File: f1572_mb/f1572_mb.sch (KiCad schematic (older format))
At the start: 24 parts, among them Q1 2N3904, SW1 power, SW2 ~reset, U1 PIC12F1572

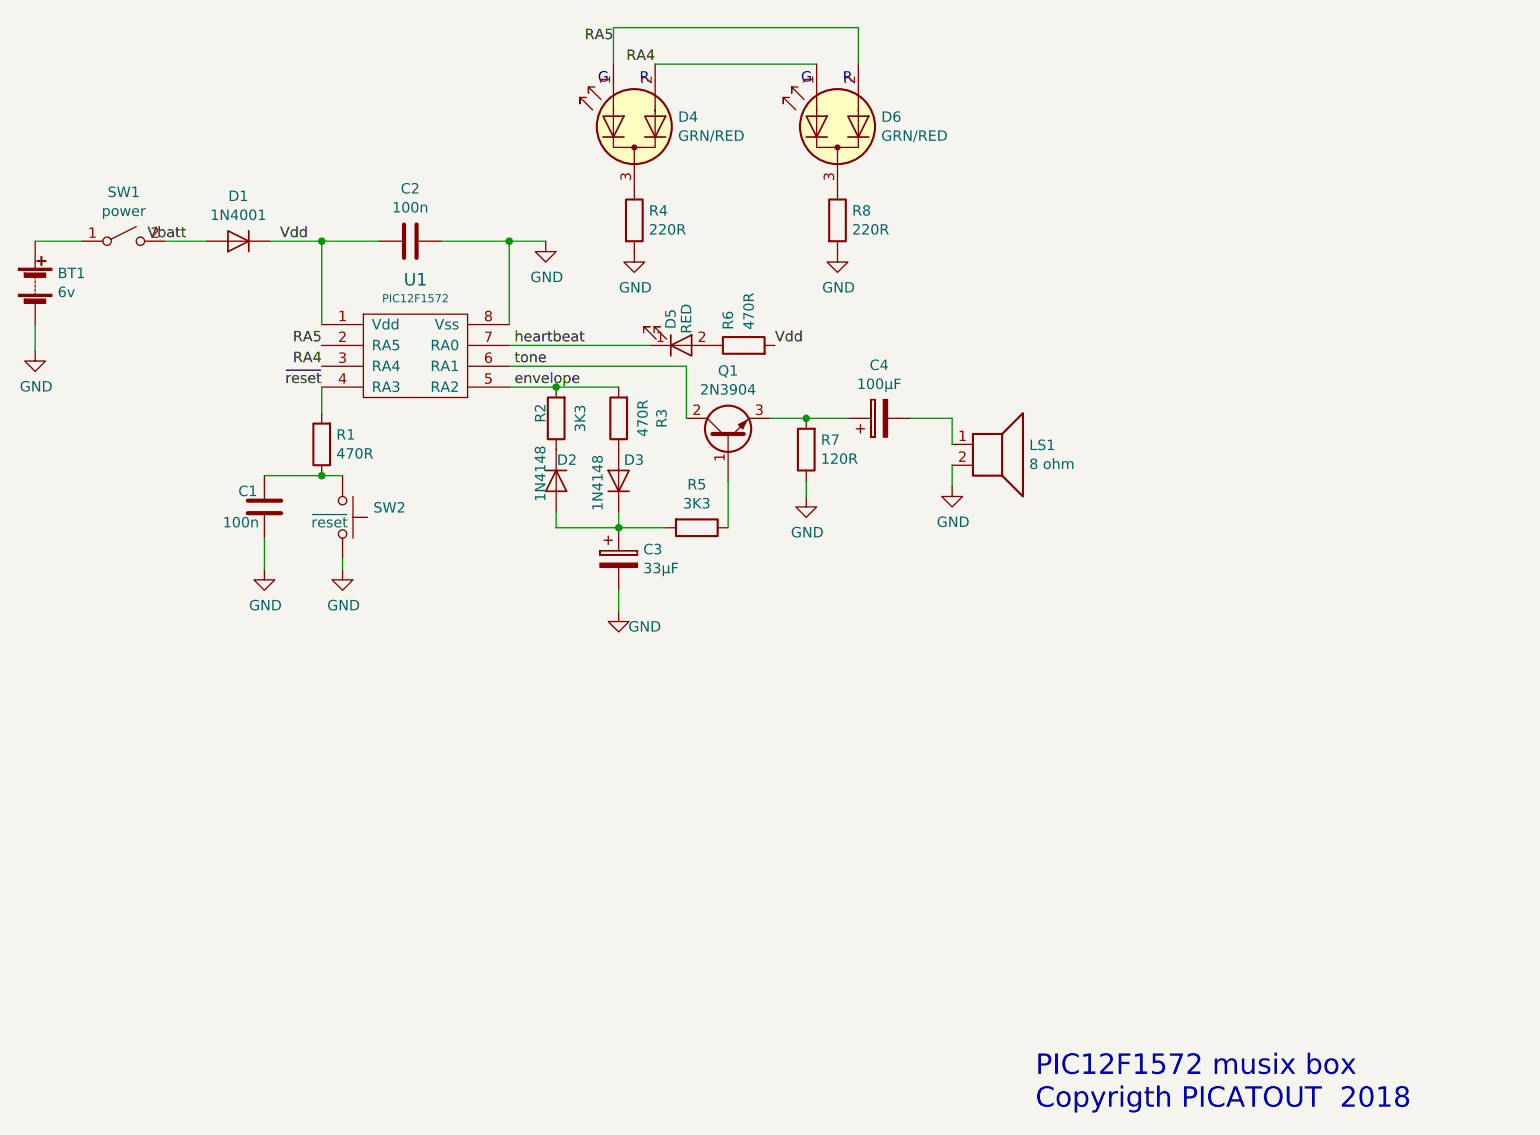
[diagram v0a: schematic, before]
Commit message: Create v2 folder and copied project file to this folder. Modified schematic
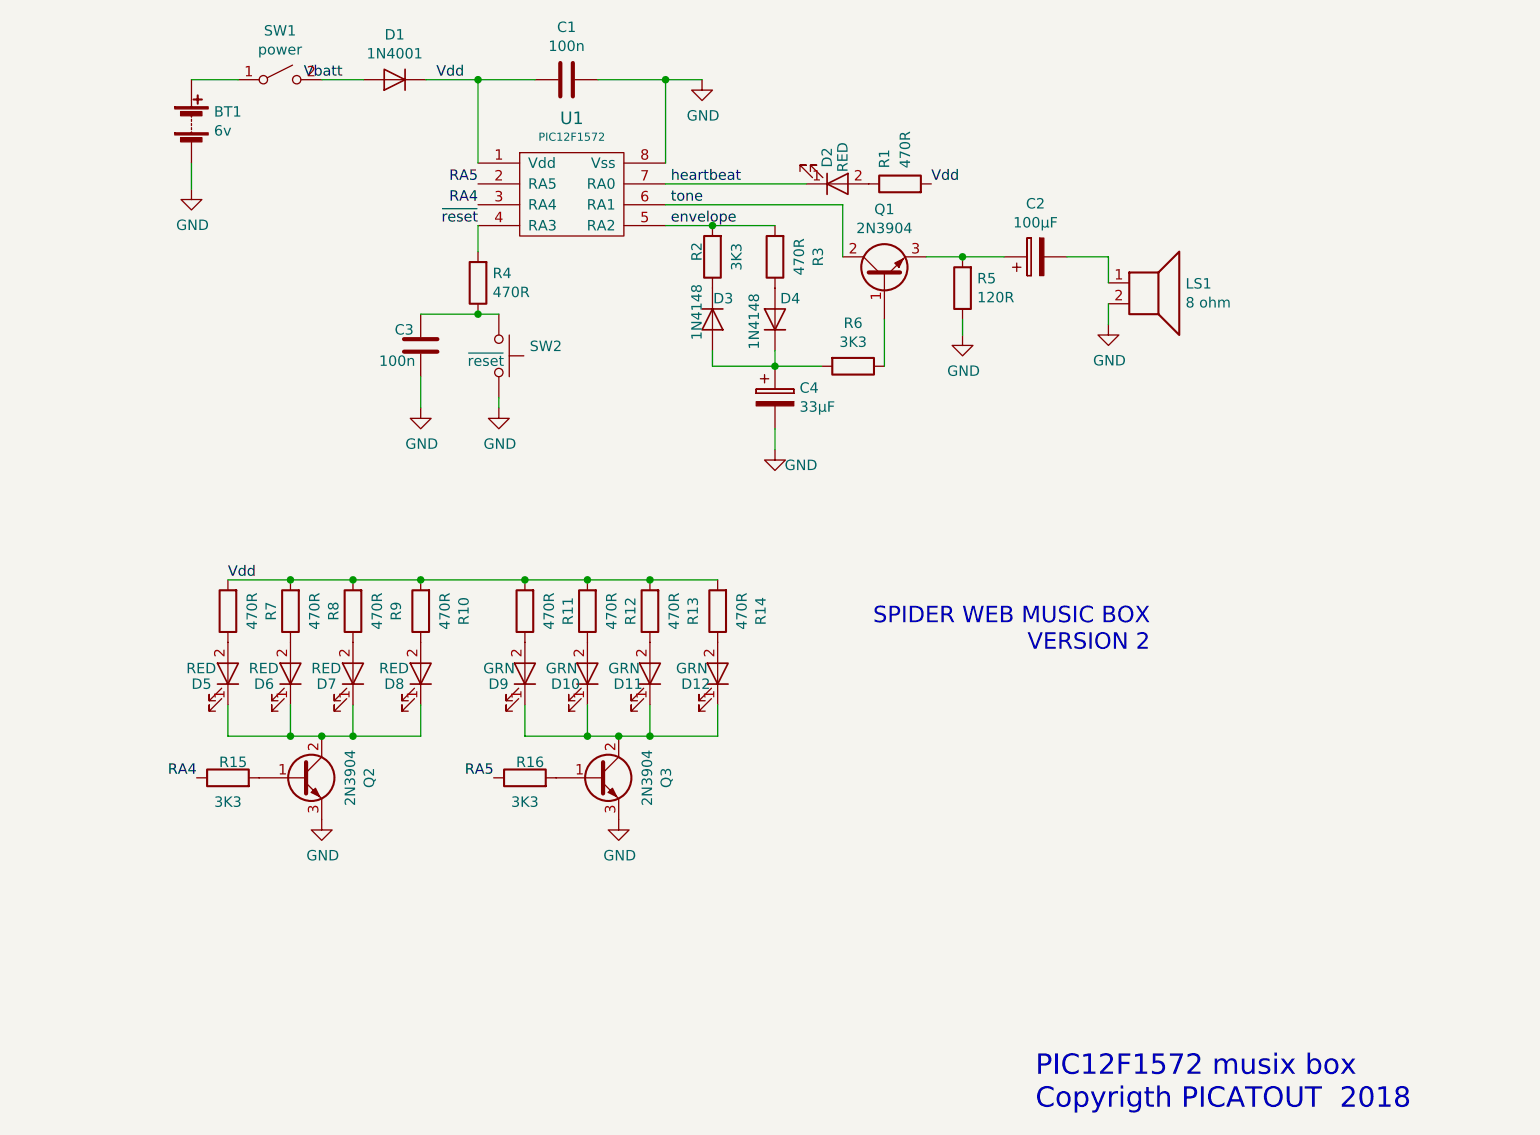
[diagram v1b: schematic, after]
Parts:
- removed D4, D6: GRN/RED, symbol device:LED_Dual_AAC
- removed R4: 220R, symbol device:R
- added D10, D11, D12, D9: GRN, symbol device:LED
- added D5, D6, D7, D8: RED, symbol device:LED
- added Q2, Q3: 2N3904, symbol device:Q_NPN_BCE
- added R10, R11, R12, R13, R14, R7, R9: 470R, symbol device:R
- added R15, R16: 3K3, symbol device:R
- R8: value 220R -> 470R
- renumbered C2 to C1, C4 to C2, C1 to C3, C3 to C4, D5 to D2, D2 to D3, D3 to D4, R6 to R1, R1 to R4, R7 to R5, R5 to R6
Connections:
- net GND: now also Q2.3 (E), Q3.3 (E); no longer R8.2
- net RA4: now also R15.1
- net RA5: now also R16.1
- net Vdd: now also R8.2, R10.2, R11.2, R12.2, R13.2, R14.2, R7.2, R9.2
- net at R8.1: now also D6.2 (A)
- new net: D5.1 (K), D6.1 (K), D7.1 (K), D8.1 (K), Q2.2 (C)
- new net: D5.2 (A), R7.1
- new net: D7.2 (A), R9.1
- new net: D8.2 (A), R10.1
- new net: D10.1 (K), D11.1 (K), D12.1 (K), D9.1 (K), Q3.2 (C)
- new net: D9.2 (A), R11.1
- new net: D10.2 (A), R12.1
- new net: D11.2 (A), R13.1
- new net: D12.2 (A), R14.1
- new net: Q2.1 (B), R15.2
- new net: Q3.1 (B), R16.2
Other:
- note added: "SPIDER WEB MUSIC BOX\nVERSION 2"
- note removed: "G\n"
- note removed: "R"
- moved on the sheet: BT1, C1, C2, C3, C4, D1, D2, D3, D4, LS1, Q1, R1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

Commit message: added png of schematic, updated readme.md
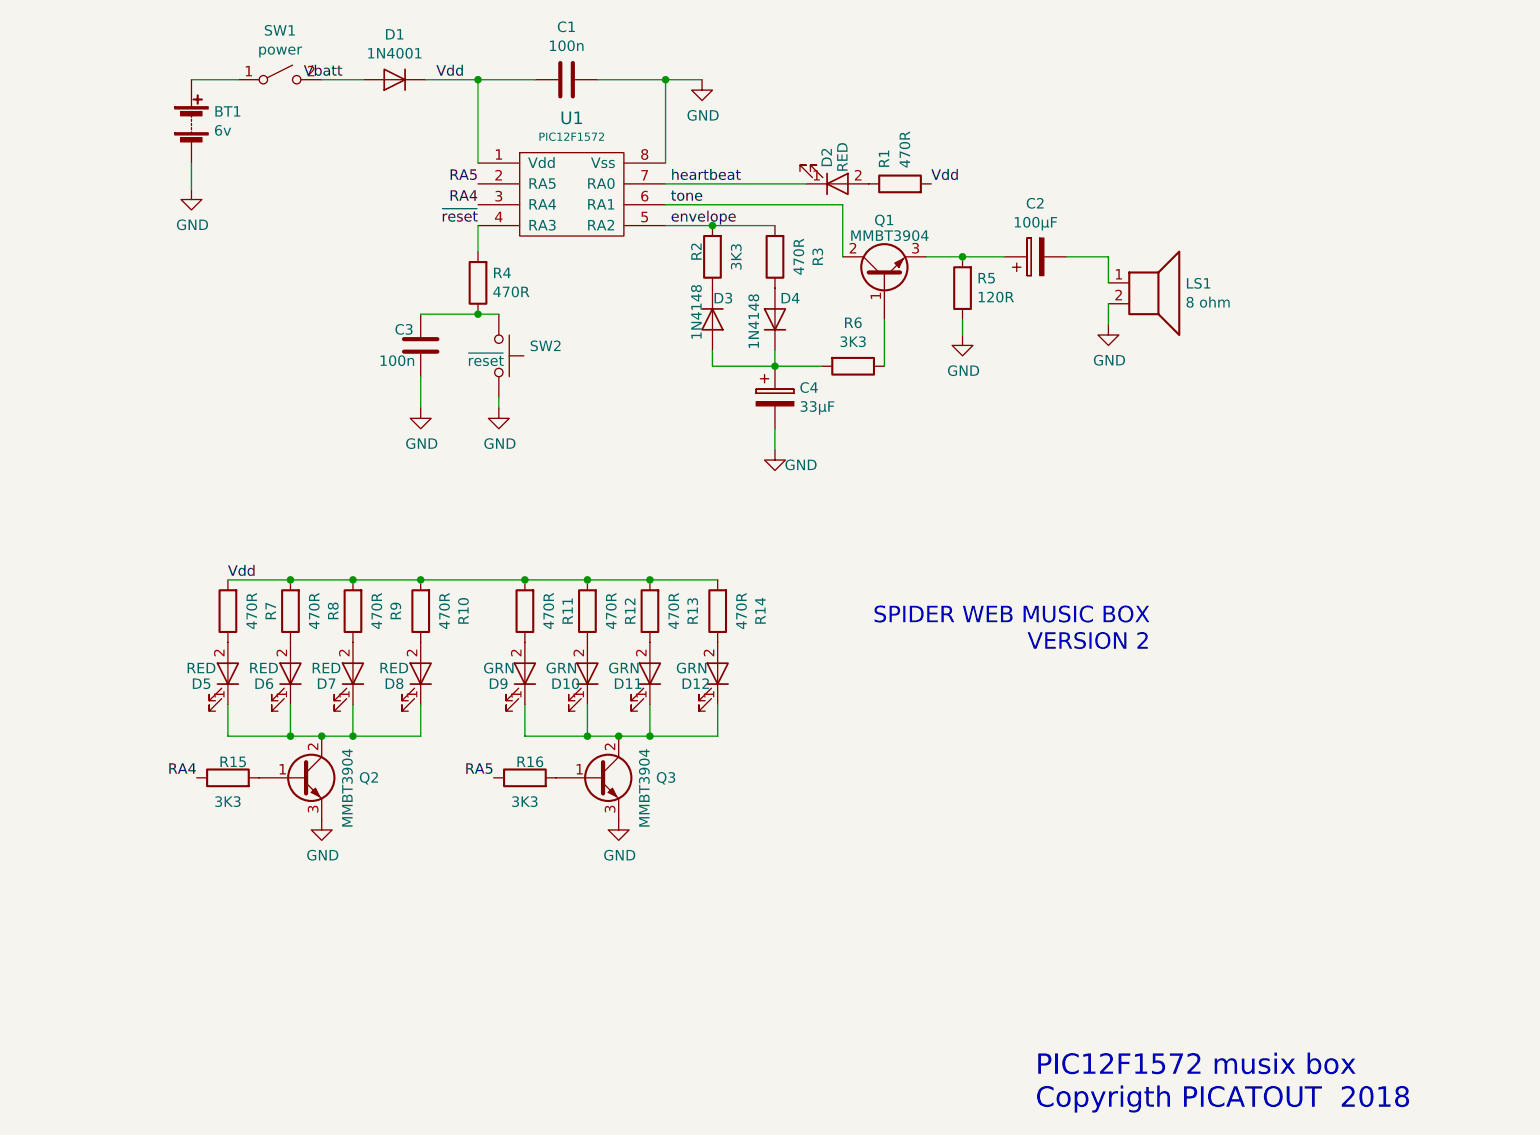
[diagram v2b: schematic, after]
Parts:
- Q1, Q2, Q3: value 2N3904 -> MMBT3904
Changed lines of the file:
@@
 U 1 1 5C074016
 P 6550 2950
-F 0 "Q1" V 6878 2950 50  0000 C CNN
-F 1 "2N3904" V 6787 2950 50  0000 C CNN
+F 0 "Q1" V 6825 2950 50  0000 C CNN
+F 1 "MMBT3904" V 6750 2925 50  0000 C CNN
 F 2 "" H 6750 3050 50  0001 C CNN
 F 3 "" H 6550 2950 50  0001 C CNN
@@
 U 1 1 5C1B7C84
 P 3750 5350
-F 0 "Q2" V 4078 5350 50  0000 C CNN
-F 1 "2N3904" V 3987 5350 50  0000 C CNN
+F 0 "Q2" H 4078 5350 50  0000 C CNN
+F 1 "MMBT3904" V 3975 5300 50  0000 C CNN
 F 2 "" H 3950 5450 50  0001 C CNN
 F 3 "" H 3750 5350 50  0001 C CNN
@@
 U 1 1 5C1B7F86
 P 5175 5350
-F 0 "Q3" V 5503 5350 50  0000 C CNN
-F 1 "2N3904" V 5412 5350 50  0000 C CNN
+F 0 "Q3" H 5503 5350 50  0000 C CNN
+F 1 "MMBT3904" V 5400 5300 50  0000 C CNN
 F 2 "" H 5375 5450 50  0001 C CNN
 F 3 "" H 5175 5350 50  0001 C CNN

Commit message: added photos project completed
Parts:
- C1, C3: footprint (none) -> Capacitors_SMD:C_0805
- D1, D3, D4, R3: footprint (none) -> Diodes_SMD:D_0805
- D10, D11, D12, D2, D5, D6, D7, D8, D9: footprint (none) -> LEDs:LED_0805
- Q1, Q2, Q3: footprint (none) -> TO_SOT_Packages_SMD:SOT-23
- R1, R10, R11, R12, R13, R14, R15, R16, R2, R5, R6, R7, R8, R9: footprint (none) -> Resistors_SMD:R_0805
- R4: footprint (none) -> Resistors_SMD:R_1206
- U1: footprint (none) -> SMD_Packages:SOIC-8-N
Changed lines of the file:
@@
 F 0 "U1" H 5050 2915 60  0000 C CNN
 F 1 "PIC12F1572" H 5050 2825 39  0000 C CNN
-F 2 "" H 5050 2350 60  0001 C CNN
+F 2 "SMD_Packages:SOIC-8-N" H 5050 2350 60  0001 C CNN
 F 3 "" H 5050 2350 60  0001 C CNN
 	1    5050 2550
@@
 F 0 "C1" V 4773 2000 50  0000 C CNN
 F 1 "100n" V 4864 2000 50  0000 C CNN
-F 2 "" H 5063 1850 50  0001 C CNN
+F 2 "Capacitors_SMD:C_0805" H 5063 1850 50  0001 C CNN
 F 3 "" H 5025 2000 50  0001 C CNN
 	1    5025 2000
@@
 F 0 "Q1" V 6825 2950 50  0000 C CNN
 F 1 "MMBT3904" V 6750 2925 50  0000 C CNN
-F 2 "" H 6750 3050 50  0001 C CNN
+F 2 "TO_SOT_Packages_SMD:SOT-23" H 6750 3050 50  0001 C CNN
 F 3 "" H 6550 2950 50  0001 C CNN
 	1    6550 2950
@@
 F 0 "R5" H 6855 2954 50  0000 R CNN
 F 1 "120R" H 6855 3045 50  0000 R CNN
-F 2 "" V 6855 3000 50  0001 C CNN
+F 2 "Resistors_SMD:R_0805" V 6855 3000 50  0001 C CNN
 F 3 "" H 6925 3000 50  0001 C CNN
 	1    6925 3000
@@
 F 0 "R6" V 6193 3375 50  0000 C CNN
 F 1 "3K3" V 6284 3375 50  0000 C CNN
-F 2 "" V 6330 3375 50  0001 C CNN
+F 2 "Resistors_SMD:R_0805" V 6330 3375 50  0001 C CNN
 F 3 "" H 6400 3375 50  0001 C CNN
 	1    6400 3375
@@
 F 0 "R3" V 5818 2850 50  0000 C CNN
 F 1 "470R" V 5909 2850 50  0000 C CNN
-F 2 "" V 5955 2850 50  0001 C CNN
+F 2 "Diodes_SMD:D_0805" V 5955 2850 50  0001 C CNN
 F 3 "" H 6025 2850 50  0001 C CNN
 	1    6025 2850
@@
 F 0 "R4" H 4530 2929 50  0000 R CNN
 F 1 "470R" H 4530 3020 50  0000 R CNN
-F 2 "" V 4530 2975 50  0001 C CNN
+F 2 "Resistors_SMD:R_1206" V 4530 2975 50  0001 C CNN
 F 3 "" H 4600 2975 50  0001 C CNN
 	1    4600 2975
@@
 F 0 "C3" H 4450 3200 50  0000 R CNN
 F 1 "100n" H 4525 3350 50  0000 R CNN
-F 2 "" H 4363 3125 50  0001 C CNN
+F 2 "Capacitors_SMD:C_0805" H 4363 3125 50  0001 C CNN
 F 3 "" H 4325 3275 50  0001 C CNN
 	1    4325 3275
@@
 F 0 "R1" H 6700 2575 50  0000 L CNN
 F 1 "470R" H 6700 2475 50  0000 L CNN
-F 2 "" V 6555 2500 50  0001 C CNN
+F 2 "Resistors_SMD:R_0805" V 6555 2500 50  0001 C CNN
 F 3 "" H 6625 2500 50  0001 C CNN
 	1    6625 2500
@@
 F 0 "D4" V 6125 3125 50  0000 R CNN
 F 1 "1N4148" H 6150 3250 50  0000 R CNN
-F 2 "" H 6025 3150 50  0001 C CNN
+F 2 "Diodes_SMD:D_0805" H 6025 3150 50  0001 C CNN
 F 3 "" H 6025 3150 50  0001 C CNN
 	1    6025 3150
@@
 F 0 "R2" V 5800 2825 50  0000 C CNN
 F 1 "3K3" V 5609 2850 50  0000 C CNN
-F 2 "" V 5655 2850 50  0001 C CNN
+F 2 "Resistors_SMD:R_0805" V 5655 2850 50  0001 C CNN
 F 3 "" H 5725 2850 50  0001 C CNN
 	1    5725 2850
@@
 F 0 "D3" V 5625 3250 50  0000 R CNN
 F 1 "1N4148" H 5825 3075 50  0000 R CNN
-F 2 "" H 5725 3150 50  0001 C CNN
+F 2 "Diodes_SMD:D_0805" H 5725 3150 50  0001 C CNN
 F 3 "" H 5725 3150 50  0001 C CNN
 	1    5725 3150
@@
 F 0 "D1" H 4200 1784 50  0000 C CNN
 F 1 "1N4001" H 4200 1875 50  0000 C CNN
-F 2 "" H 4200 2000 50  0001 C CNN
+F 2 "Diodes_SMD:D_0805" H 4200 2000 50  0001 C CNN
 F 3 "" H 4200 2000 50  0001 C CNN
 	1    4200 2000
@@
 F 0 "D2" V 6275 2325 50  0000 L CNN
 F 1 "RED" V 6350 2300 50  0000 L CNN
-F 2 "" H 6325 2500 50  0001 C CNN
+F 2 "LEDs:LED_0805" H 6325 2500 50  0001 C CNN
 F 3 "" H 6325 2500 50  0001 C CNN
 	1    6325 2500
@@
 F 0 "D5" V 3350 4675 50  0000 L CNN
 F 1 "RED" V 3425 4650 50  0000 L CNN
-F 2 "" H 3400 4850 50  0001 C CNN
+F 2 "LEDs:LED_0805" H 3400 4850 50  0001 C CNN
 F 3 "" H 3400 4850 50  0001 C CNN
 	1    3400 4850
@@
 F 0 "D6" V 3650 4675 50  0000 L CNN
 F 1 "RED" V 3725 4650 50  0000 L CNN
-F 2 "" H 3700 4850 50  0001 C CNN
+F 2 "LEDs:LED_0805" H 3700 4850 50  0001 C CNN
 F 3 "" H 3700 4850 50  0001 C CNN
 	1    3700 4850
@@
 F 0 "D7" V 3950 4675 50  0000 L CNN
 F 1 "RED" V 4025 4650 50  0000 L CNN
-F 2 "" H 4000 4850 50  0001 C CNN
+F 2 "LEDs:LED_0805" H 4000 4850 50  0001 C CNN
 F 3 "" H 4000 4850 50  0001 C CNN
 	1    4000 4850
@@
 F 0 "D8" V 4275 4675 50  0000 L CNN
 F 1 "RED" V 4350 4650 50  0000 L CNN
-F 2 "" H 4325 4850 50  0001 C CNN
+F 2 "LEDs:LED_0805" H 4325 4850 50  0001 C CNN
 F 3 "" H 4325 4850 50  0001 C CNN
 	1    4325 4850
@@
 F 0 "D9" V 4775 4675 50  0000 L CNN
 F 1 "GRN" V 4850 4650 50  0000 L CNN
-F 2 "" H 4825 4850 50  0001 C CNN
+F 2 "LEDs:LED_0805" H 4825 4850 50  0001 C CNN
 F 3 "" H 4825 4850 50  0001 C CNN
 	1    4825 4850
@@
 F 0 "D10" V 5075 4675 50  0000 L CNN
 F 1 "GRN" V 5150 4650 50  0000 L CNN
-F 2 "" H 5125 4850 50  0001 C CNN
+F 2 "LEDs:LED_0805" H 5125 4850 50  0001 C CNN
 F 3 "" H 5125 4850 50  0001 C CNN
 	1    5125 4850
@@
 F 0 "D11" V 5375 4675 50  0000 L CNN
 F 1 "GRN" V 5450 4650 50  0000 L CNN
-F 2 "" H 5425 4850 50  0001 C CNN
+F 2 "LEDs:LED_0805" H 5425 4850 50  0001 C CNN
 F 3 "" H 5425 4850 50  0001 C CNN
 	1    5425 4850
@@
 F 0 "D12" V 5700 4675 50  0000 L CNN
 F 1 "GRN" V 5775 4650 50  0000 L CNN
-F 2 "" H 5750 4850 50  0001 C CNN
+F 2 "LEDs:LED_0805" H 5750 4850 50  0001 C CNN
 F 3 "" H 5750 4850 50  0001 C CNN
 	1    5750 4850
@@
 F 0 "Q2" H 4078 5350 50  0000 C CNN
 F 1 "MMBT3904" V 3975 5300 50  0000 C CNN
-F 2 "" H 3950 5450 50  0001 C CNN
+F 2 "TO_SOT_Packages_SMD:SOT-23" H 3950 5450 50  0001 C CNN
 F 3 "" H 3750 5350 50  0001 C CNN
 	1    3750 5350
@@
 F 0 "Q3" H 5503 5350 50  0000 C CNN
 F 1 "MMBT3904" V 5400 5300 50  0000 C CNN
-F 2 "" H 5375 5450 50  0001 C CNN
+F 2 "TO_SOT_Packages_SMD:SOT-23" H 5375 5450 50  0001 C CNN
 F 3 "" H 5175 5350 50  0001 C CNN
 	1    5175 5350
@@
 F 0 "R7" V 3193 4550 50  0000 C CNN
 F 1 "470R" V 3284 4550 50  0000 C CNN
-F 2 "" V 3330 4550 50  0001 C CNN
+F 2 "Resistors_SMD:R_0805" V 3330 4550 50  0001 C CNN
 F 3 "" H 3400 4550 50  0001 C CNN
 	1    3400 4550
@@
 F 0 "R8" V 3493 4550 50  0000 C CNN
 F 1 "470R" V 3584 4550 50  0000 C CNN
-F 2 "" V 3630 4550 50  0001 C CNN
+F 2 "Resistors_SMD:R_0805" V 3630 4550 50  0001 C CNN
 F 3 "" H 3700 4550 50  0001 C CNN
 	1    3700 4550
@@
 F 0 "R9" V 3793 4550 50  0000 C CNN
 F 1 "470R" V 3884 4550 50  0000 C CNN
-F 2 "" V 3930 4550 50  0001 C CNN
+F 2 "Resistors_SMD:R_0805" V 3930 4550 50  0001 C CNN
 F 3 "" H 4000 4550 50  0001 C CNN
 	1    4000 4550
@@
 F 0 "R10" V 4118 4550 50  0000 C CNN
 F 1 "470R" V 4209 4550 50  0000 C CNN
-F 2 "" V 4255 4550 50  0001 C CNN
+F 2 "Resistors_SMD:R_0805" V 4255 4550 50  0001 C CNN
 F 3 "" H 4325 4550 50  0001 C CNN
 	1    4325 4550
@@
 F 0 "R11" V 4618 4550 50  0000 C CNN
 F 1 "470R" V 4709 4550 50  0000 C CNN
-F 2 "" V 4755 4550 50  0001 C CNN
+F 2 "Resistors_SMD:R_0805" V 4755 4550 50  0001 C CNN
 F 3 "" H 4825 4550 50  0001 C CNN
 	1    4825 4550
@@
 F 0 "R12" V 4918 4550 50  0000 C CNN
 F 1 "470R" V 5009 4550 50  0000 C CNN
-F 2 "" V 5055 4550 50  0001 C CNN
+F 2 "Resistors_SMD:R_0805" V 5055 4550 50  0001 C CNN
 F 3 "" H 5125 4550 50  0001 C CNN
 	1    5125 4550
@@
 F 0 "R13" V 5218 4550 50  0000 C CNN
 F 1 "470R" V 5309 4550 50  0000 C CNN
-F 2 "" V 5355 4550 50  0001 C CNN
+F 2 "Resistors_SMD:R_0805" V 5355 4550 50  0001 C CNN
 F 3 "" H 5425 4550 50  0001 C CNN
 	1    5425 4550
@@
 F 0 "R14" V 5543 4550 50  0000 C CNN
 F 1 "470R" V 5634 4550 50  0000 C CNN
-F 2 "" V 5680 4550 50  0001 C CNN
+F 2 "Resistors_SMD:R_0805" V 5680 4550 50  0001 C CNN
 F 3 "" H 5750 4550 50  0001 C CNN
 	1    5750 4550
@@
 F 0 "R15" V 3475 5325 50  0000 C CNN
 F 1 "3K3" V 3284 5350 50  0000 C CNN
-F 2 "" V 3330 5350 50  0001 C CNN
+F 2 "Resistors_SMD:R_0805" V 3330 5350 50  0001 C CNN
 F 3 "" H 3400 5350 50  0001 C CNN
 	1    3400 5350
@@
 F 0 "R16" V 4900 5325 50  0000 C CNN
 F 1 "3K3" V 4709 5350 50  0000 C CNN
-F 2 "" V 4755 5350 50  0001 C CNN
+F 2 "Resistors_SMD:R_0805" V 4755 5350 50  0001 C CNN
 F 3 "" H 4825 5350 50  0001 C CNN
 	1    4825 5350
